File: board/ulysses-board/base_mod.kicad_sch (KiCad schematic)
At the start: 33 parts, among them J3 RS-232, J4 LC display, Q2 BC548, Q3 BC548, SW10 Config, SW3 UP, SW4 Ri, SW5 DN, SW6 Le, SW7 OK, SW8 EJ0, SW9 EJ1, U4 Firmware, U5 MAX3232, U6 Config, U7 MCP23008, U8 BOB-12009

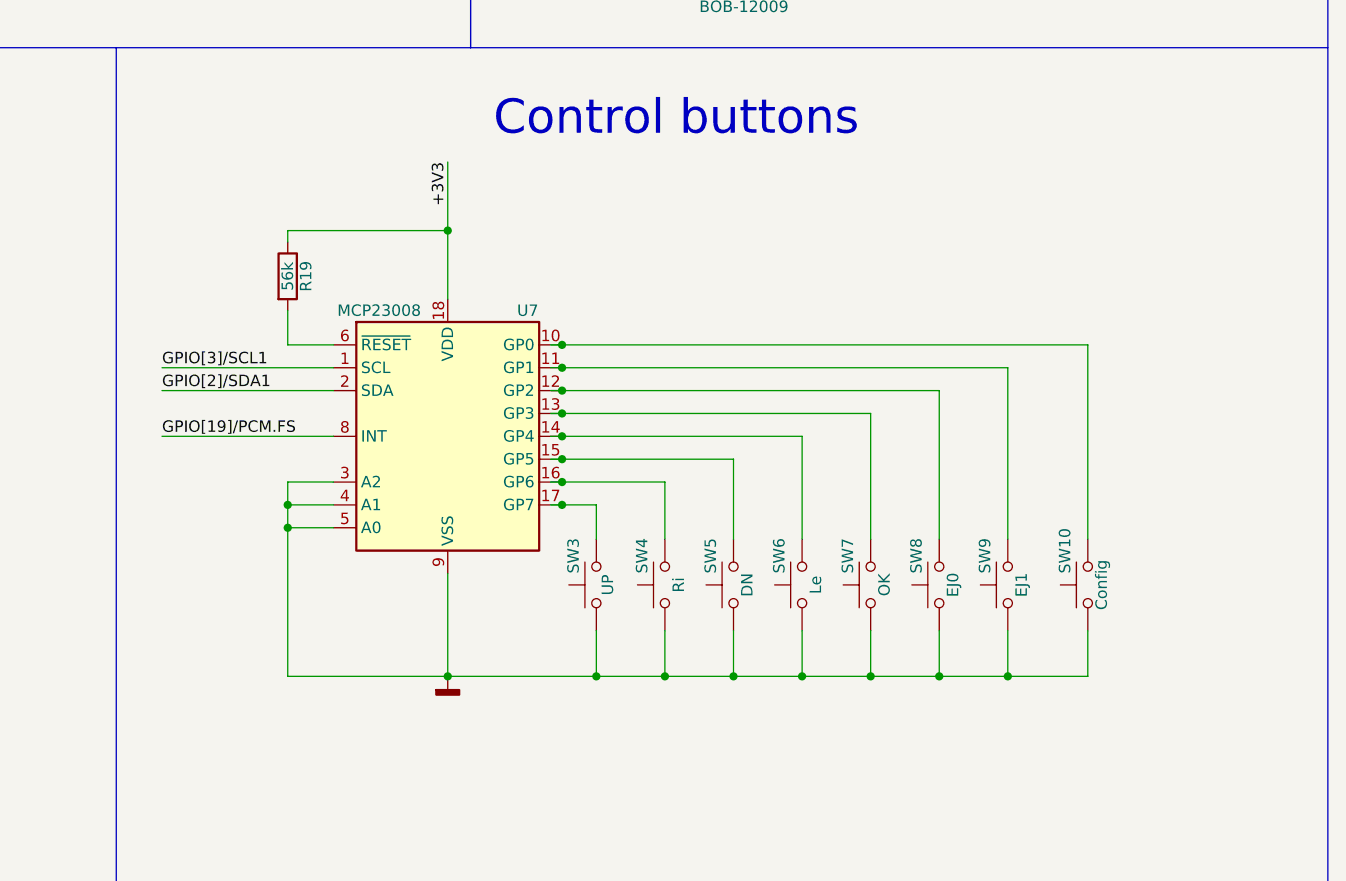
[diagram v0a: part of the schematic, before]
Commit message: Make some minor fixes.
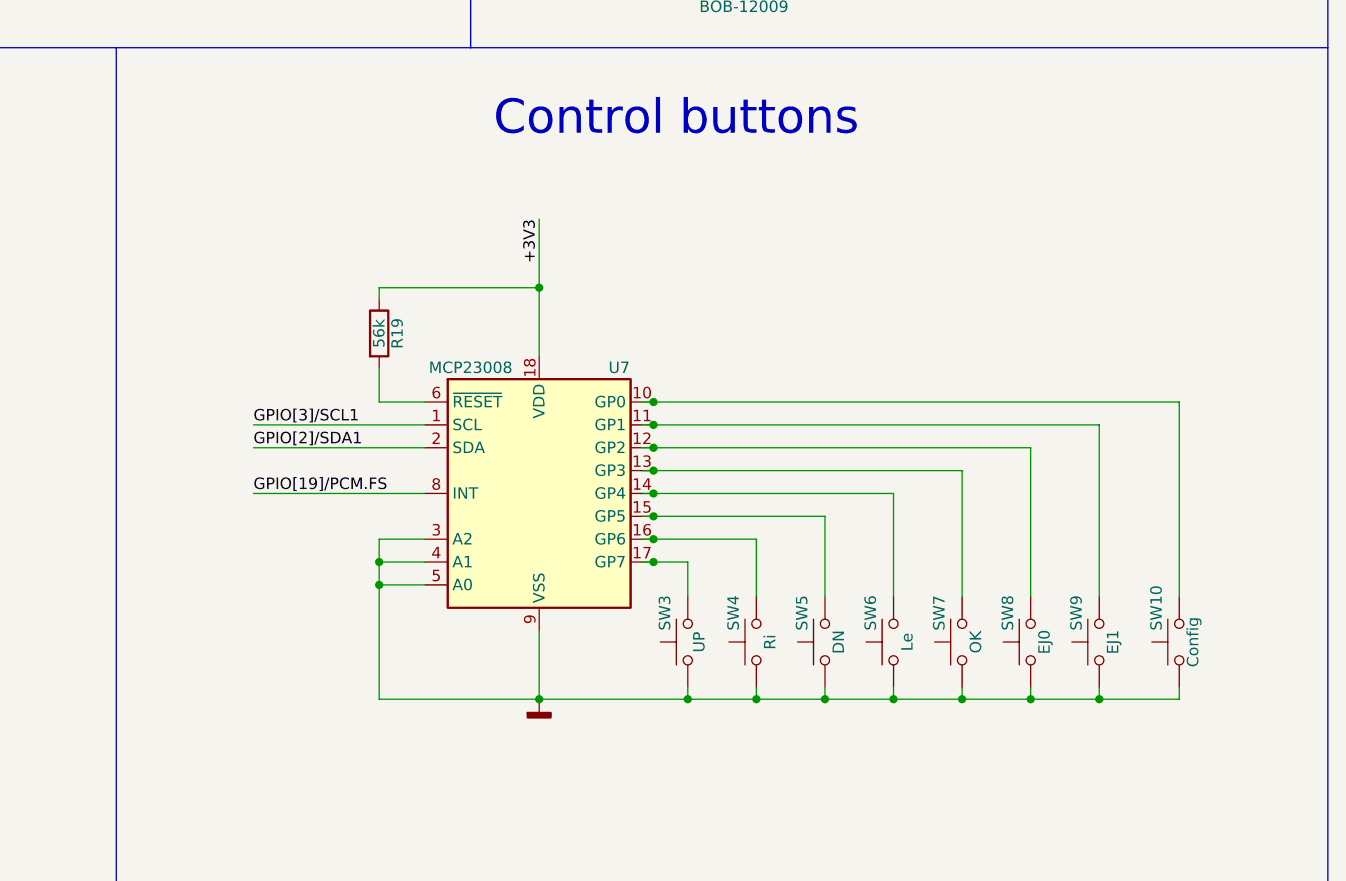
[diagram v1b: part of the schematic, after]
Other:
- moved on the sheet: R19, SW10, SW3, SW4, SW5, SW6, SW7, SW8, SW9, U7
